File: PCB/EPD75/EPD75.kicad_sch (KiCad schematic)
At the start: 115 parts, among them J1 Conn_01x26, J10 TF_PUSH, J11 Reset, J12 TC2030-USB-NL-DS, J3 RELAY, J4 BTN1, J5 USB-C-Socket-V, J6 BTN2, J7 USB-C-Socket-V, J8 PWR, Q1 BSS138, U2 ESP32-S3-MINI-1, U3 MD8942, U8 G3VM-41GR8

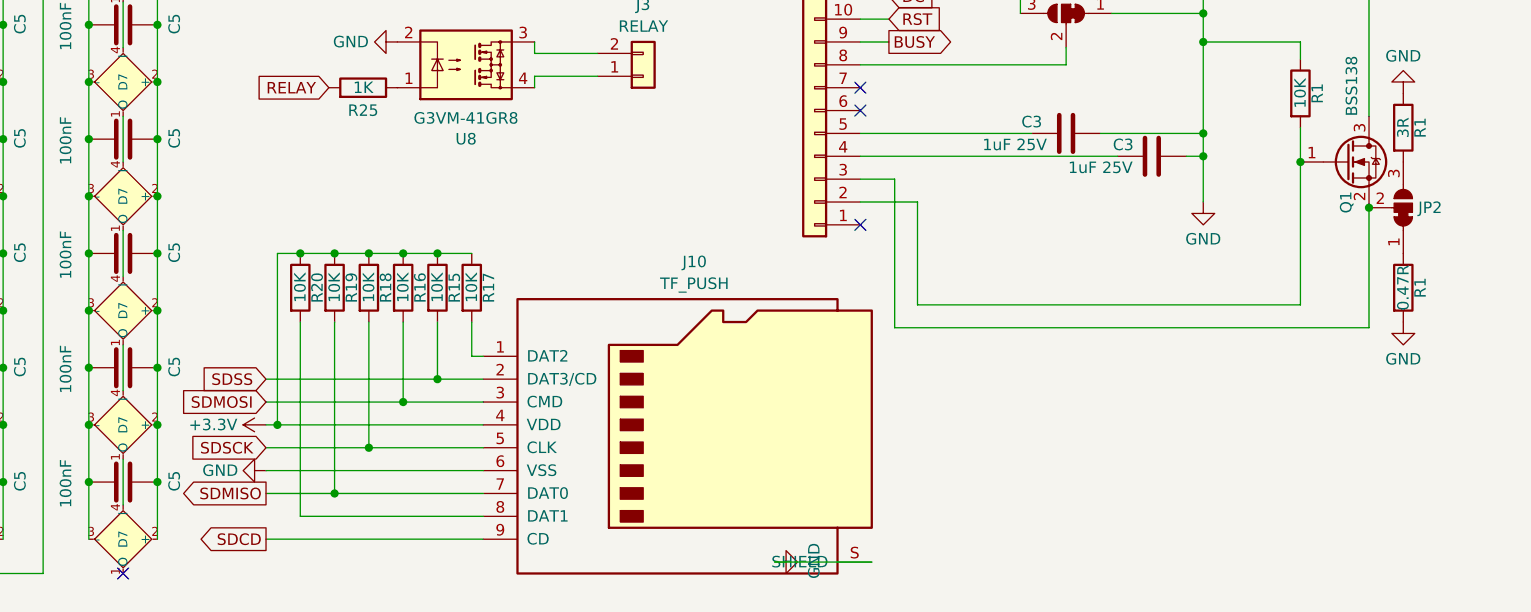
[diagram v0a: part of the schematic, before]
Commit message: Tidy
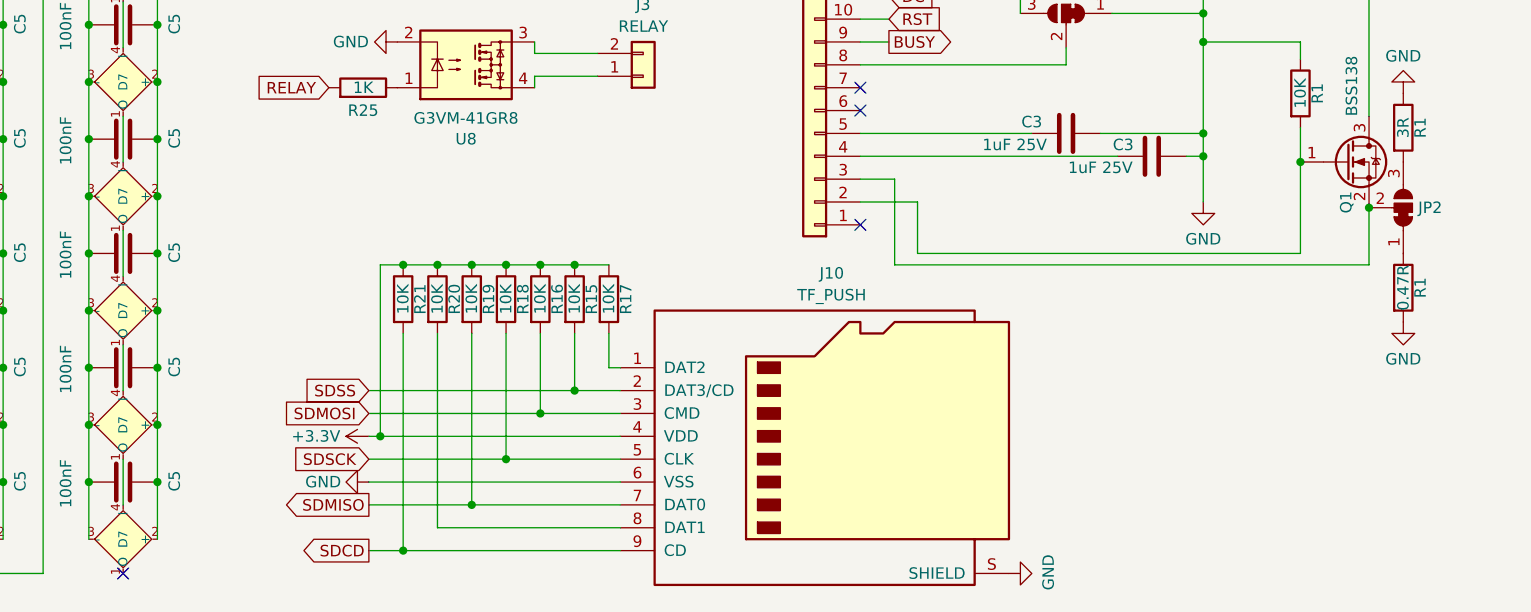
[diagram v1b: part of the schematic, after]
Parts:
- added R21: 10K, RevK:R_0402, symbol Device:R
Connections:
- net +3.3V: now also R21.1
- net SDCD: now also R21.2
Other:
- moved on the sheet: J10, R15, R16, R17, R18, R19, R20
